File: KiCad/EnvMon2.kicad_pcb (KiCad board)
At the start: 2 copper layers, 34 x 37 mm, 32 parts, among them J1 USB-C, J2 DC, J3 TEMP, M1 OLED1.5-RGB, U1 LMR16006+FB, U2 SCD41, U3 FT231XQ, U4 DS18B20, U5 ESP32-PICO-MINI-02, U6 QR

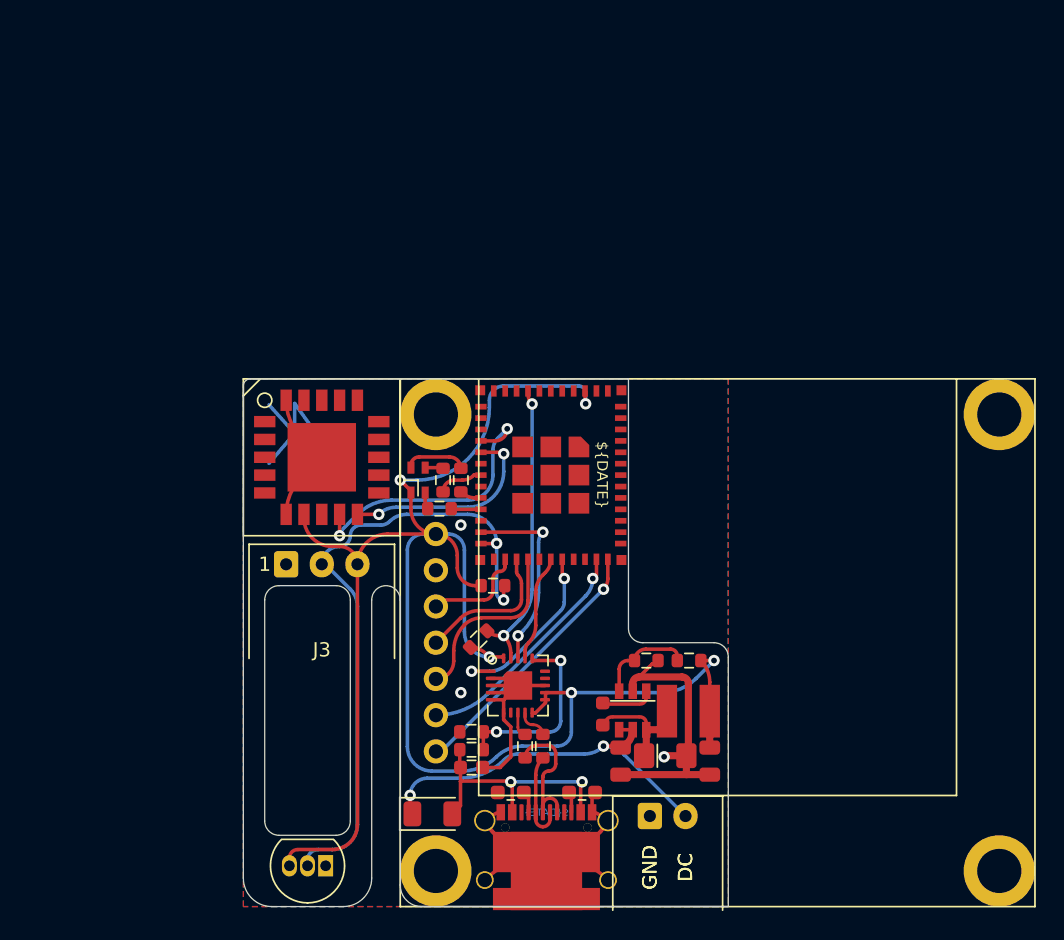
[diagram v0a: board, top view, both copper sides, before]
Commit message: New case
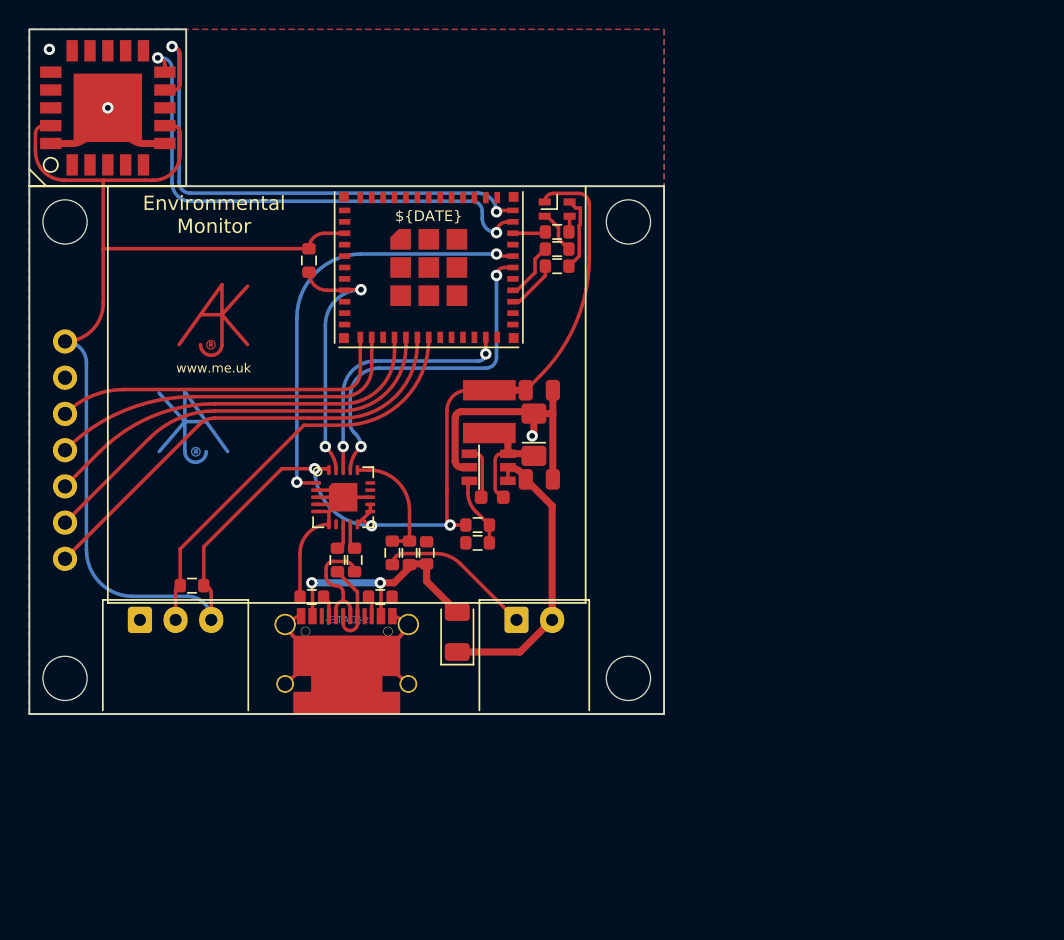
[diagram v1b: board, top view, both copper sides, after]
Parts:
- removed U6: QR, RevK:QR-ENVMON
- added Logo2: AJK, RevK:AJK, F.Cu at (113.5, 72.0)
- R12: value 4k7 -> 10k
- R13: value 10k -> 4k7
- R3, R4: footprint Resistor_SMD:R_0603_1608Metric_Pad0.98x0.95mm_HandSolder -> RevK:R_0603
- U4: value DS18B20 -> ESP32-PICO-MINI-02; footprint Package_TO_SOT_THT:TO-92_Inline -> RevK:ESP32-PICO-MINI-02
- U5: value ESP32-PICO-MINI-02 -> QR; footprint RevK:ESP32-PICO-MINI-02 -> RevK:QR-ENVMON; moved to B.Cu
- moved U4 42.6 mm to (128.0, 68.7), turned to 0 degrees
- moved M1 29.3 mm to (144.5, 63.0)
- moved U2 28.7 mm to (105.5, 57.5), turned to 90 degrees
- moved C3 28.6 mm to (135.8, 77.3), turned to 0 degrees
- moved R12 26.2 mm to (119.6, 68.2), turned to -90 degrees
- moved L1 25.2 mm to (132.2, 78.8), turned to 90 degrees
- moved D1 24.3 mm to (135.4, 80.4), turned to 90 degrees
- moved D3 21.4 mm to (137.0, 64.6), turned to 180 degrees
- moved C2 20.6 mm to (135.8, 83.5), turned to 0 degrees
- moved R13 20.4 mm to (111.4, 91.0), turned to 0 degrees
- moved R9 20.0 mm to (137.0, 67.4), turned to 180 degrees
- moved U5 19.8 mm to (122.2, 97.0), turned to 0 degrees
- moved U1 19.8 mm to (132.2, 82.7), turned to 90 degrees
- moved R4 19.7 mm to (124.6, 91.8)
- moved J1 19.6 mm to (122.2, 100.0)
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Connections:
- R12 pad 2: TEMP -> EN
- R13 pad 1: +3V3 -> TEMP
- R13 pad 2: EN -> +3V3
- U2 pad 19: unconnected-(U2-Pad19) -> +3V3
- U4 pad 2: TEMP -> GND
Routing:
- net CO2-SDA: track 14.6 -> 37.1 mm
- net CO2-SCL: track 20.1 -> 38.6 mm
- net O: track 13.0 -> 30.5 mm
- net I: track 7.43 -> 24.5 mm, vias 0 -> 2
- net OLED-MOSI: track 7.25 -> 24.2 mm
- net TEMP: track 45.9 -> 29.5 mm, vias 2 -> 0
- net OLED-SCLK: track 10.2 -> 25.7 mm
- net OLED-CS0: track 12.8 -> 27.9 mm
- net OLED-RST: track 18.6 -> 31.9 mm, vias 1 -> 0
- net OLED-DC: track 16.5 -> 29.9 mm, vias 1 -> 0
- net GND: track 28.6 -> 36.2 mm
- net DC: track 26.0 -> 19.1 mm, vias 2 -> 0
- net +3V3: track 131.5 -> 136.5 mm, vias 5 -> 3
- net Net-(R10-Pad2): track 13.4 -> 8.51 mm, vias 2 -> 0
- net BOOT: track 13.6 -> 18.0 mm
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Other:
- board size 34 x 37 mm -> 44.5 x 48 mm
- board text added: "DC 4V-60V"
- board text added: "DS18B20"
- board text removed: "DC"
- board text removed: "GND"
